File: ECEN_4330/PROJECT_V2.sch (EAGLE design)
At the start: 31 parts, among them IC1 74AS573N

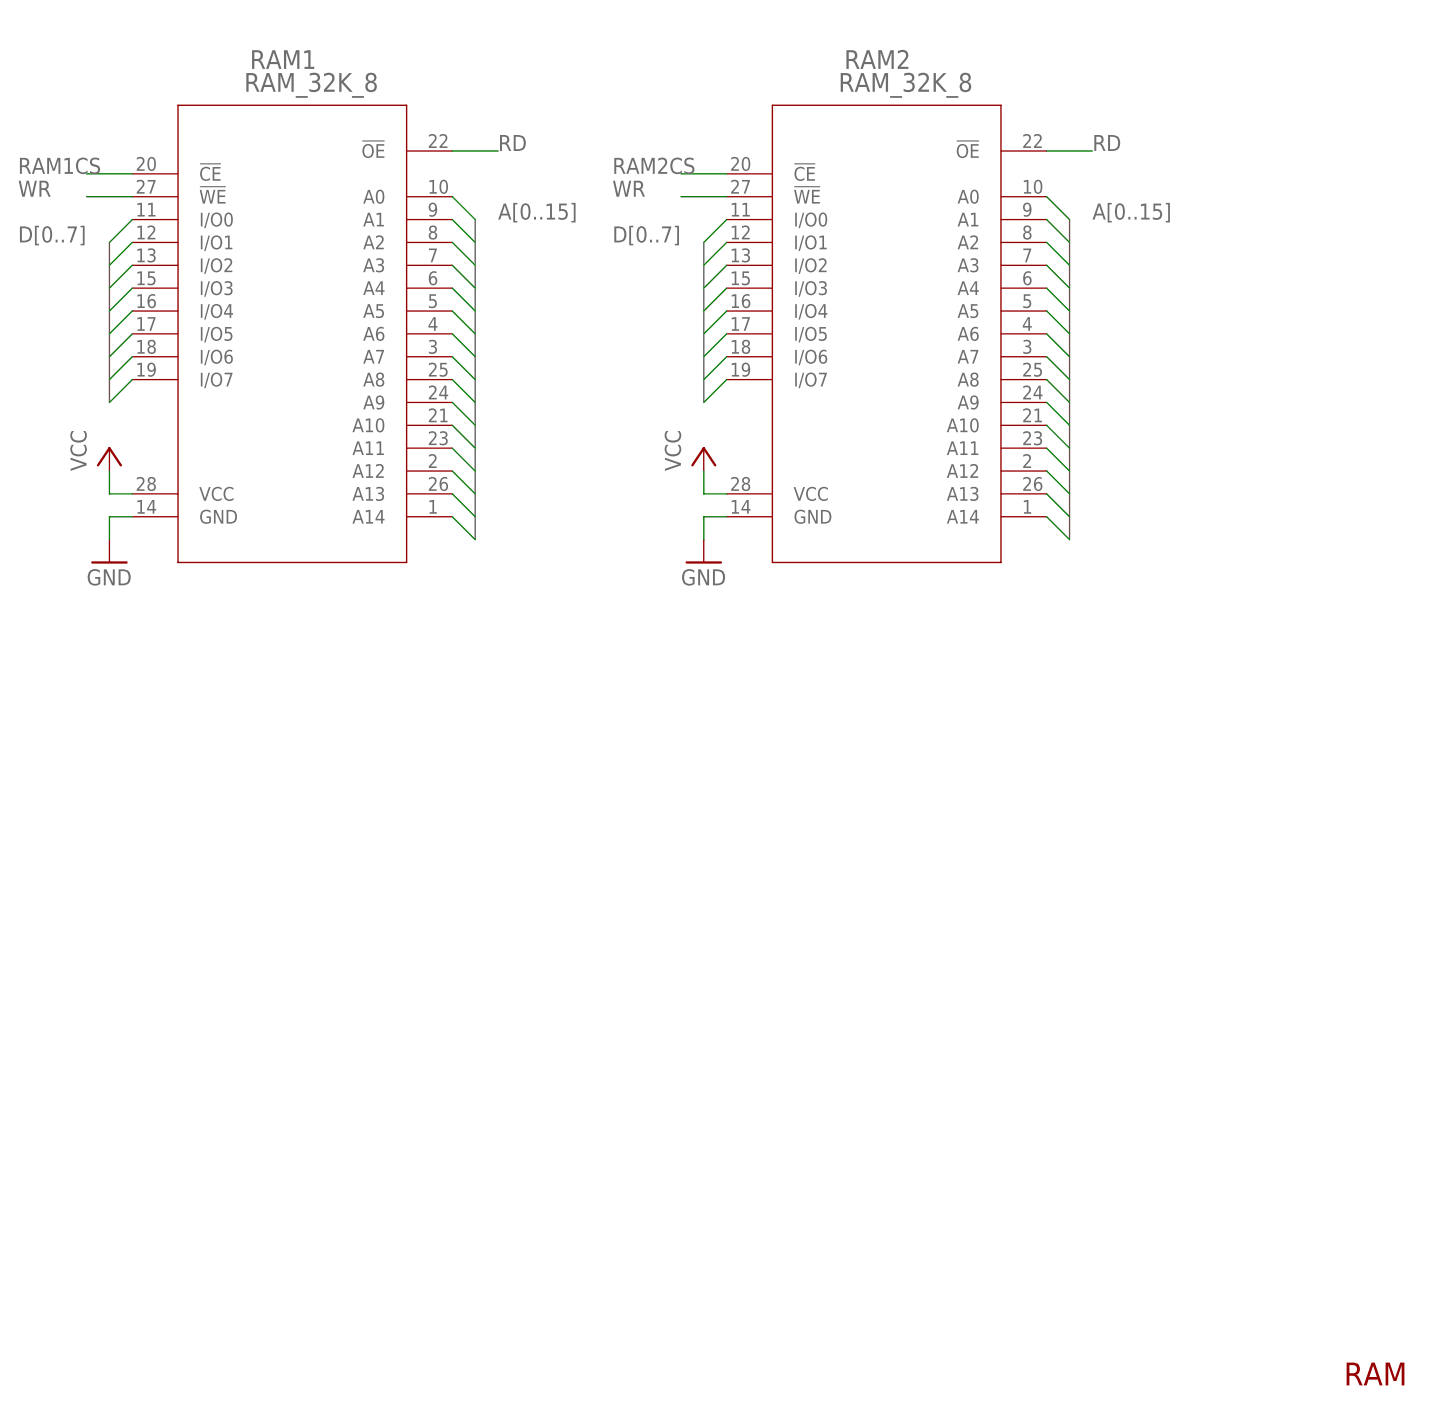
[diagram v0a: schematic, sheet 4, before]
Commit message: Final design before hierarchiel block
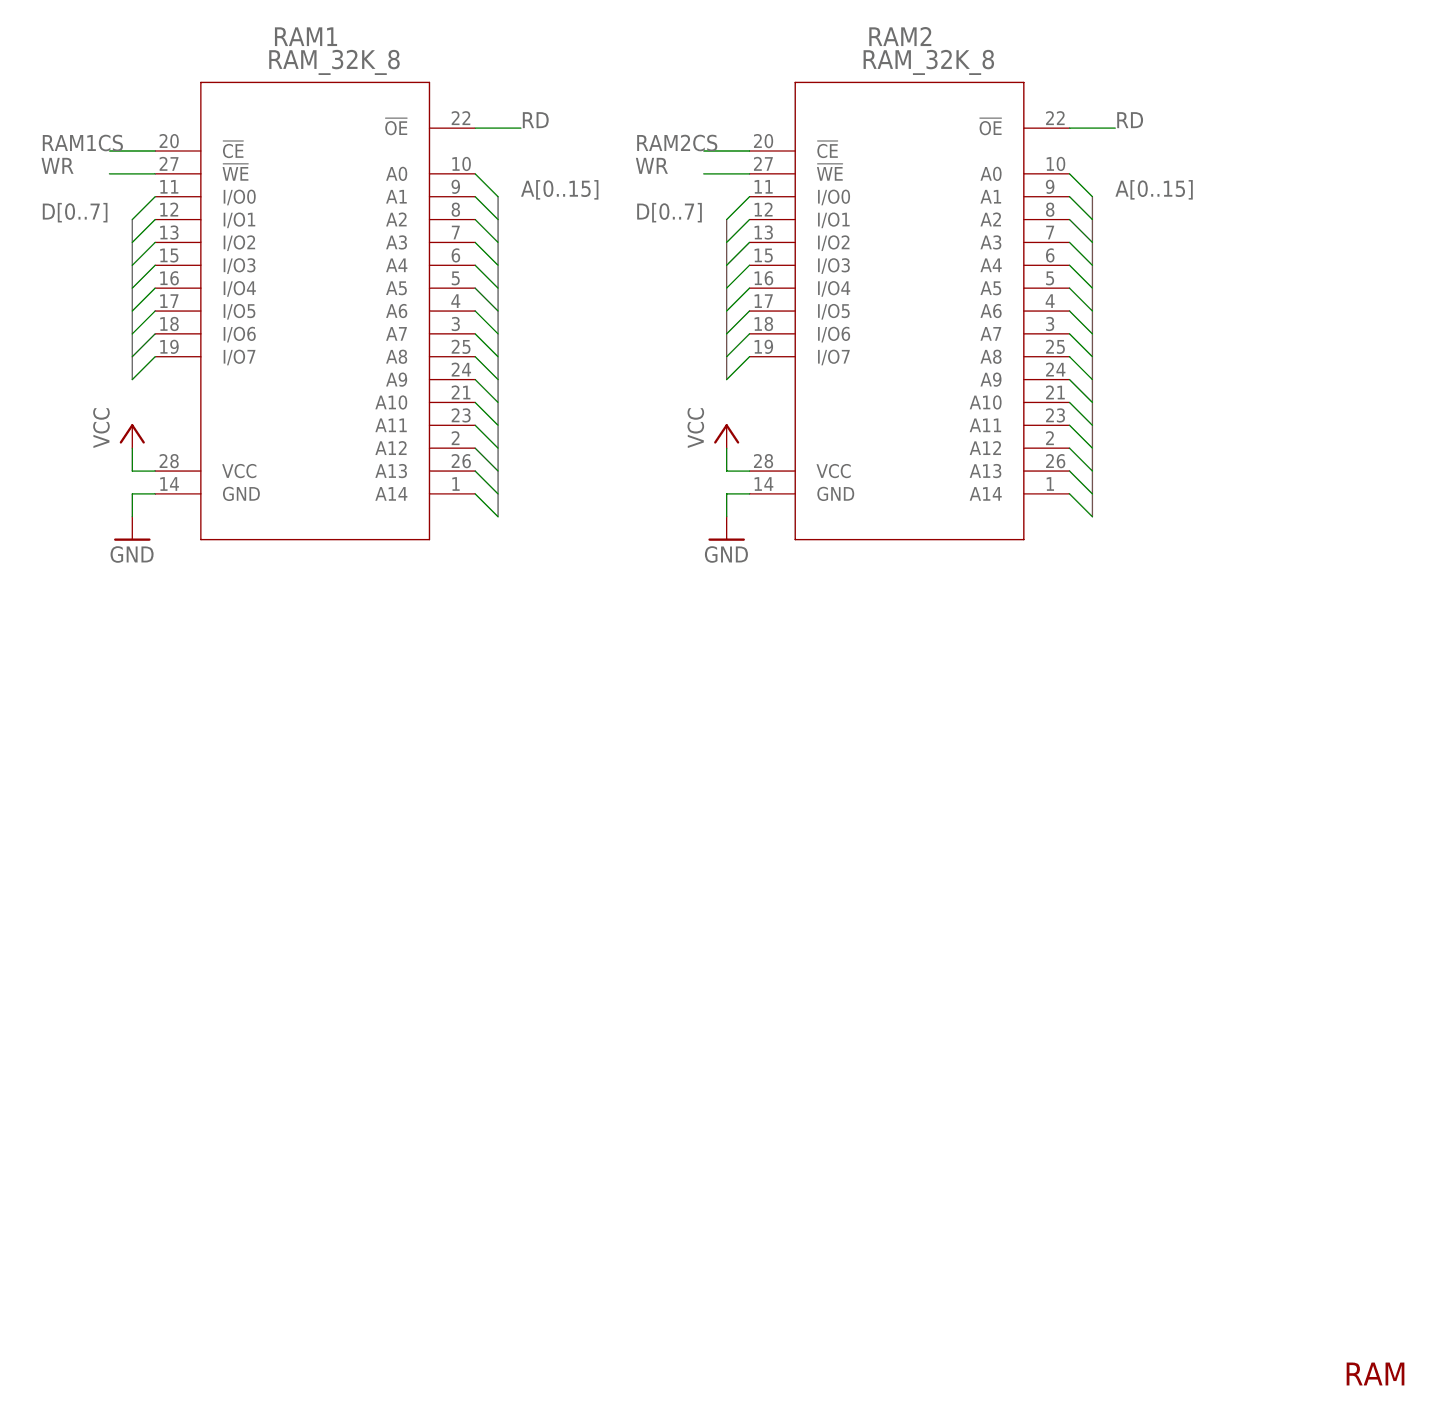
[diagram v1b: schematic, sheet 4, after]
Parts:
- added R11: (no value), resistor:R-US_0204/7
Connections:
- new net N$30: J1.3, LED1.A, S1.S
- new net N$48: S1.O
- new net N$49: LED1.C, R11.2
- net GND: now also J1.1, J1.2, R11.1
- net VCC: now also S1.P
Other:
- moved on the sheet: J1, LED1, RAM1, RAM2, RTC, S1
